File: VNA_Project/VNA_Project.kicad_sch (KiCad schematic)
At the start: 0 parts

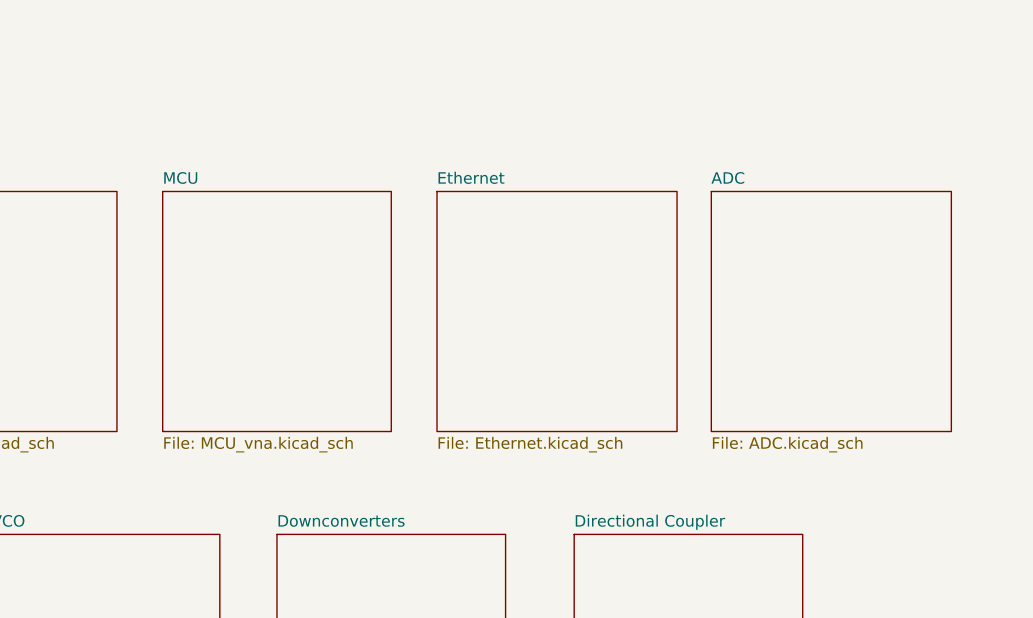
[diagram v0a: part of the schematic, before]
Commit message: footprints + initial layout shape
footprints + initial layout shape
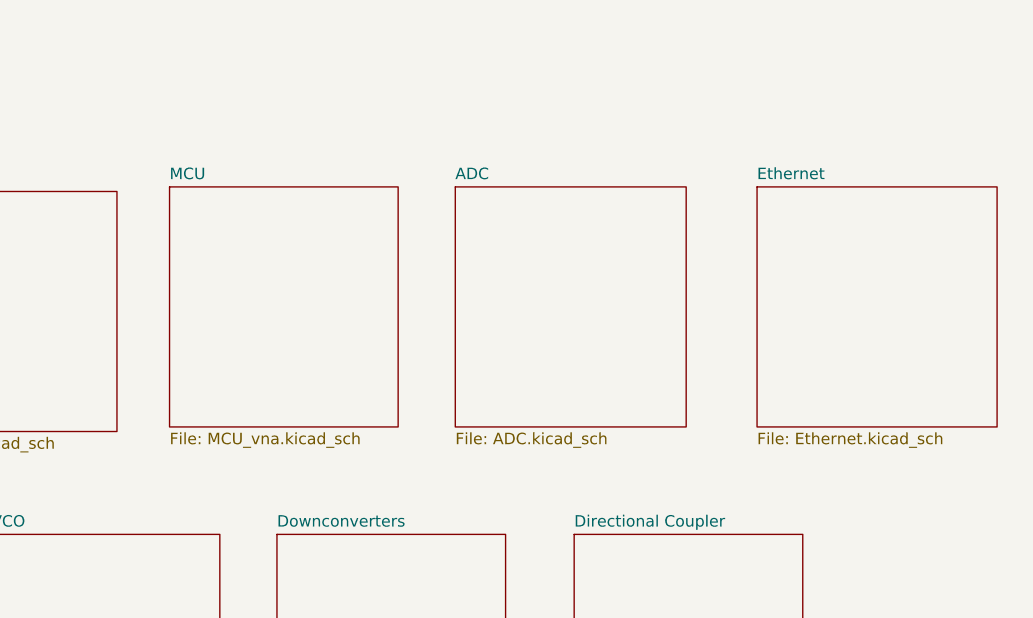
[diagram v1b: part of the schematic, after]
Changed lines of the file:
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@@
 	)
 	(sheet
-		(at 129.54 66.04)
+		(at 165.1 65.532)
 		(size 26.67 26.67)
 		(exclude_from_sim no)
@@
 		)
 		(property "Sheetname" "Ethernet"
-			(at 129.54 65.3284 0)
+			(at 165.1 64.8204 0)
 			(effects
 				(font
@@
 		)
 		(property "Sheetfile" "Ethernet.kicad_sch"
-			(at 129.54 93.2946 0)
-			(effects
-				(font
-					(size 1.27 1.27)
-				)
-				(justify left top)
-			)
-		)
-		(instances
-			(project "VNA_Project"
-				(path "/8b9c6944-c5f7-4a92-a452-dc4fa5f3924d"
-					(page "10")
+			(at 165.1 92.7866 0)
+			(effects
+				(font
+					(size 1.27 1.27)
+				)
+				(justify left top)
+			)
+		)
+		(instances
+			(project "VNA_Project"
+				(path "/8b9c6944-c5f7-4a92-a452-dc4fa5f3924d"
+					(page "5")
 				)
 			)
@@
 			(project "VNA_Project"
 				(path "/8b9c6944-c5f7-4a92-a452-dc4fa5f3924d"
-					(page "5")
-				)
-			)
-		)
-	)
-	(sheet
-		(at 99.06 66.04)
+					(page "8")
+				)
+			)
+		)
+	)
+	(sheet
+		(at 99.822 65.532)
 		(size 25.4 26.67)
 		(exclude_from_sim no)
@@
 		)
 		(property "Sheetname" "MCU"
-			(at 99.06 65.3284 0)
+			(at 99.822 64.8204 0)
 			(effects
 				(font
@@
 		)
 		(property "Sheetfile" "MCU_vna.kicad_sch"
-			(at 99.06 93.2946 0)
+			(at 99.822 92.7866 0)
+			(effects
+				(font
+					(size 1.27 1.27)
+				)
+				(justify left top)
+			)
+		)
+		(instances
+			(project "VNA_Project"
+				(path "/8b9c6944-c5f7-4a92-a452-dc4fa5f3924d"
+					(page "3")
+				)
+			)
+		)
+	)
+	(sheet
+		(at 131.572 65.532)
+		(size 25.654 26.67)
+		(exclude_from_sim no)
+		(in_bom yes)
+		(on_board yes)
+		(dnp no)
+		(fields_autoplaced yes)
+		(stroke
+			(width 0.1524)
+			(type solid)
+		)
+		(fill
+			(color 0 0 0 0.0000)
+		)
+		(property "Sheetname" "ADC"
+			(at 131.572 64.8204 0)
+			(effects
+				(font
+					(size 1.27 1.27)
+				)
+				(justify left bottom)
+			)
+		)
+		(property "Sheetfile" "ADC.kicad_sch"
+			(at 131.572 92.7866 0)
 			(effects
 				(font
@@
 				(path "/8b9c6944-c5f7-4a92-a452-dc4fa5f3924d"
 					(page "4")
-				)
-			)
-		)
-	)
-	(sheet
-		(at 160.02 66.04)
-		(size 26.67 26.67)
-		(exclude_from_sim no)
-		(in_bom yes)
-		(on_board yes)
-		(dnp no)
-		(fields_autoplaced yes)
-		(stroke
-			(width 0.1524)
-			(type solid)
-		)
-		(fill
-			(color 0 0 0 0.0000)
-		)
-		(property "Sheetname" "ADC"
-			(at 160.02 65.3284 0)
-			(effects
-				(font
-					(size 1.27 1.27)
-				)
-				(justify left bottom)
-			)
-		)
-		(property "Sheetfile" "ADC.kicad_sch"
-			(at 160.02 93.2946 0)
-			(effects
-				(font
-					(size 1.27 1.27)
-				)
-				(justify left top)
-			)
-		)
-		(instances
-			(project "VNA_Project"
-				(path "/8b9c6944-c5f7-4a92-a452-dc4fa5f3924d"
-					(page "6")
 				)
 			)
@@
 			(project "VNA_Project"
 				(path "/8b9c6944-c5f7-4a92-a452-dc4fa5f3924d"
-					(page "3")
+					(page "6")
 				)
 			)
@@
 			(project "VNA_Project"
 				(path "/8b9c6944-c5f7-4a92-a452-dc4fa5f3924d"
-					(page "8")
-				)
-			)
+					(page "7")
+				)
+			)
